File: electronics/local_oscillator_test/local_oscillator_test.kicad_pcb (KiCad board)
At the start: 2 copper layers, 4 parts, among them U1 CE3520K3

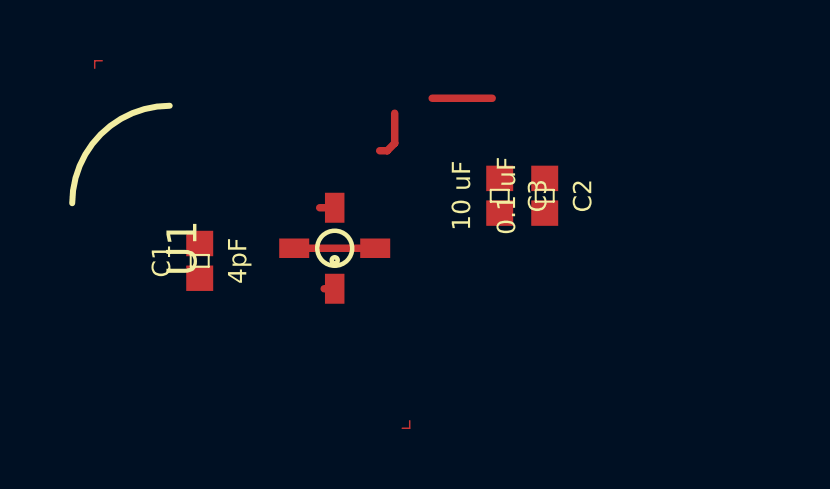
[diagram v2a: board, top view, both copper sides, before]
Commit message: Phage propagation!
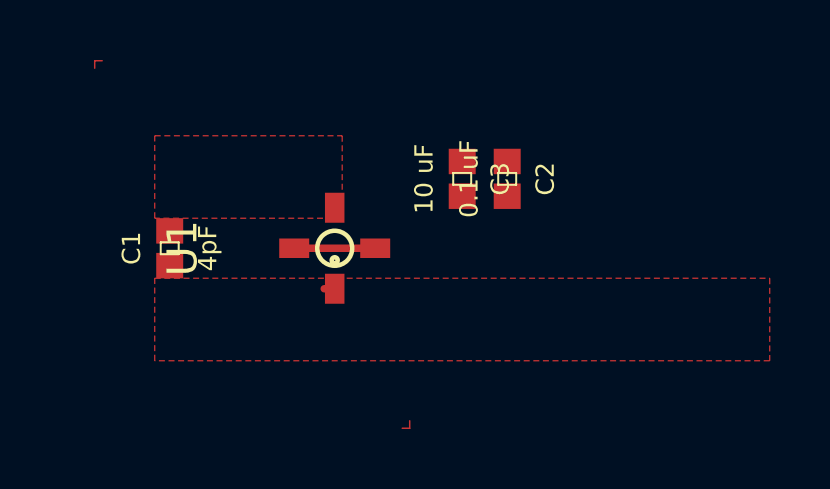
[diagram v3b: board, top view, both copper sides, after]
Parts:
- moved C2 1.37 mm to (28.8, 16.4)
- moved C3 1.37 mm to (27.2, 16.4)
- moved C1 1.08 mm to (17.5, 18.8)
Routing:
- net (no net): track 4.60 -> 1.00 mm
- added copper zone on F.Cu, net /GATE
- added copper zone on F.Cu, net /OSC1
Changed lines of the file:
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@@
   (general
     (thickness 1.6)
-    (drawings 1)
-    (tracks 12)
+    (drawings 0)
+    (tracks 8)
     (zones 0)
     (modules 4)
@@
   )
   (module 0402 (layer F.Cu)
-    (at 28.5 17 270)
+    (at 27.25 16.4368 270)
     (descr "GENERIC 1005 (0402) PACKAGE")
     (tags "GENERIC 1005 (0402) PACKAGE")
@@
   )
   (module 0402 (layer F.Cu)
-    (at 30 17 270)
+    (at 28.75 16.4368 270)
     (descr "GENERIC 1005 (0402) PACKAGE")
     (tags "GENERIC 1005 (0402) PACKAGE")
@@
   )
   (module 0402 (layer F.Cu)
-    (at 18.5 19.17088 90)
+    (at 17.5 18.75 90)
     (descr "GENERIC 1005 (0402) PACKAGE")
     (tags "GENERIC 1005 (0402) PACKAGE")
@@
       (net 1 /OSC1) (solder_mask_margin 0.1016))
   )
-  (gr_arc (start 17.5 17.25) (end 17.5 14) (angle -90) (layer F.SilkS) (width 0.2))
   (segment (start 15 12.75) (end 15 12.5) (width 0.05) (layer F.Cu) (net 0))
   (segment (start 15 12.5) (end 15.25 12.5) (width 0.05) (layer F.Cu) (net 0))
   (segment (start 25.5 24.5) (end 25.5 24.75) (width 0.05) (layer F.Cu) (net 0))
   (segment (start 25.5 24.75) (end 25.25 24.75) (width 0.05) (layer F.Cu) (net 0))
-  (segment (start 24.5 15.5) (end 24.75 15.5) (width 0.25) (layer F.Cu) (net 0))
-  (segment (start 24.75 15.5) (end 25 15.25) (width 0.25) (layer F.Cu) (net 0))
-  (segment (start 25 15.25) (end 25 14.25) (width 0.25) (layer F.Cu) (net 0))
-  (segment (start 26.25 13.75) (end 28.25 13.75) (width 0.25) (layer F.Cu) (net 0))
-  (segment (start 22.85 17.4) (end 22.5 17.4) (width 0.25) (layer F.Cu) (net 1))
   (segment (start 23 20.1) (end 22.65 20.1) (width 0.25) (layer F.Cu) (net 3))
+  (segment (start 22.97912 20.07912) (end 23 20.1) (width 0.25) (layer F.Cu) (net 3))
   (segment (start 22.4 18.75) (end 24.35 18.75) (width 0.25) (layer F.Cu) (net 4))
   (segment (start 21.65 18.75) (end 22.4 18.75) (width 0.25) (layer F.Cu) (net 4))
+  (zone (net 1) (net_name /OSC1) (layer F.Cu) (hatch edge 0.508)
+    (connect_pads yes (clearance 0))
+    (min_thickness 0.254)
+    (fill yes (arc_segments 16) (thermal_gap 0) (thermal_bridge_width 0))
+    (polygon
+      (pts
+        (xy 23.25 17.75) (xy 17 17.75) (xy 17 15) (xy 23.25 15)
+      )
+    )
+  )
+  (zone (net 3) (net_name /GATE) (layer F.Cu) (hatch edge 0.508)
+    (connect_pads yes (clearance 0))
+    (min_thickness 0.254)
+    (fill yes (arc_segments 16) (thermal_gap 0) (thermal_bridge_width 0))
+    (polygon
+      (pts
+        (xy 37.5 22.5) (xy 17 22.5) (xy 17 19.75) (xy 37.5 19.75)
+      )
+    )
+  )
 )
